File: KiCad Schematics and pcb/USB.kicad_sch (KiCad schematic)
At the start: 22 parts, among them IC4 TPS25730DREFR, J7 USB_C_Receptacle_USB2.0_16P, U1 TVS2200DRV

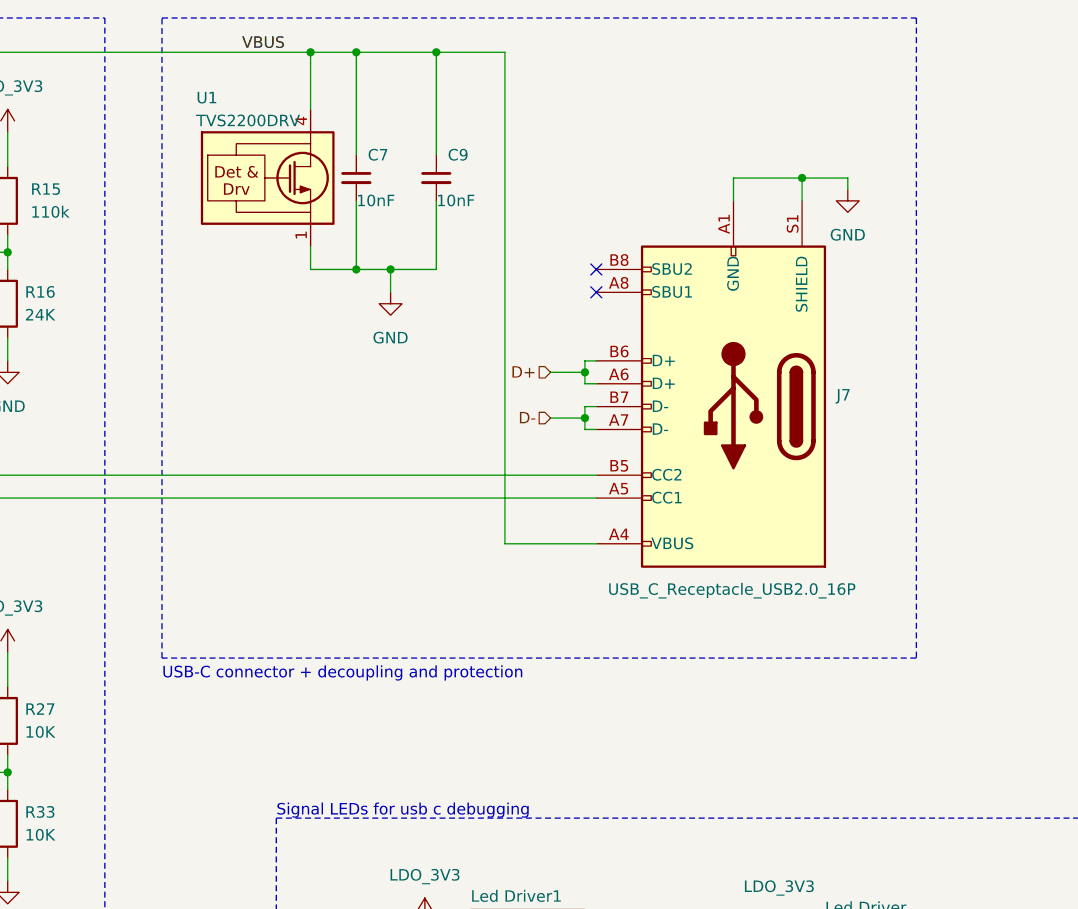
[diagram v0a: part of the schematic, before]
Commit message: 0.2
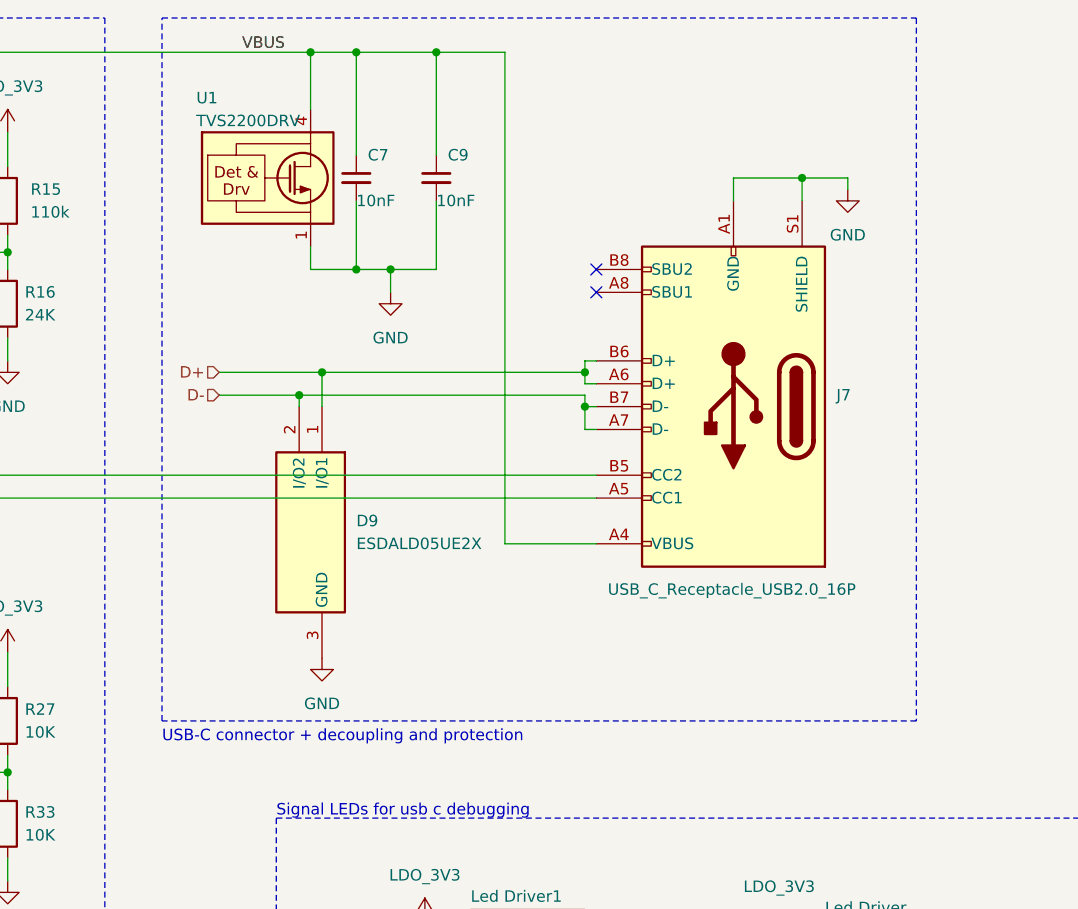
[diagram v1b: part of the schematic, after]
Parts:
- added D9: ESDALD05UE2X, SOT95P240X115-3N, symbol ComponentSearch:ESDALD05UE2X
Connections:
- net D+: now also D9.1 (I/O1)
- net D-: now also D9.2 (I/O2)
- net GND: now also D9.3 (GND)
